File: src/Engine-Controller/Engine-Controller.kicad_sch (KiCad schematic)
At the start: 21 parts, among them J1 Jumper_NO, J2 Jumper_NO, P3 3220-20-0200-00, U1 STM32H750VBTx, Y1 ECS-240-18-33-JGN-TR

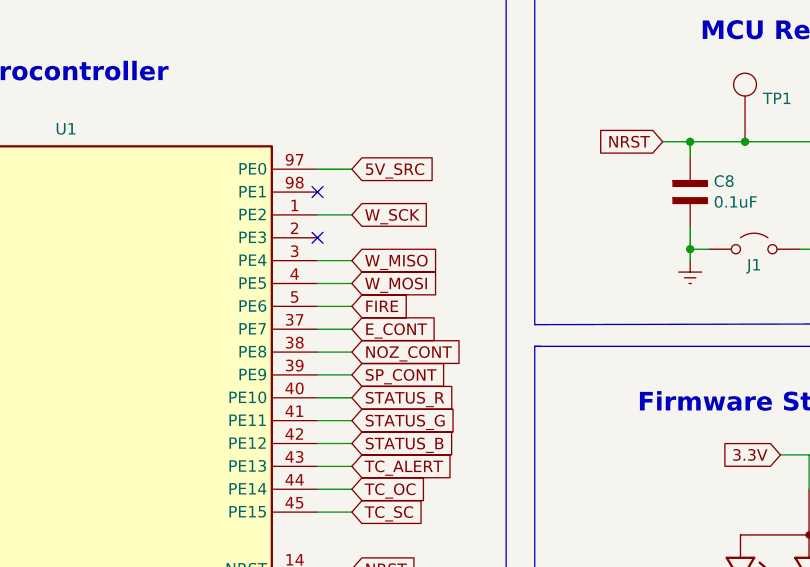
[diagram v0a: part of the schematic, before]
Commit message: completed rev 5.0 layout
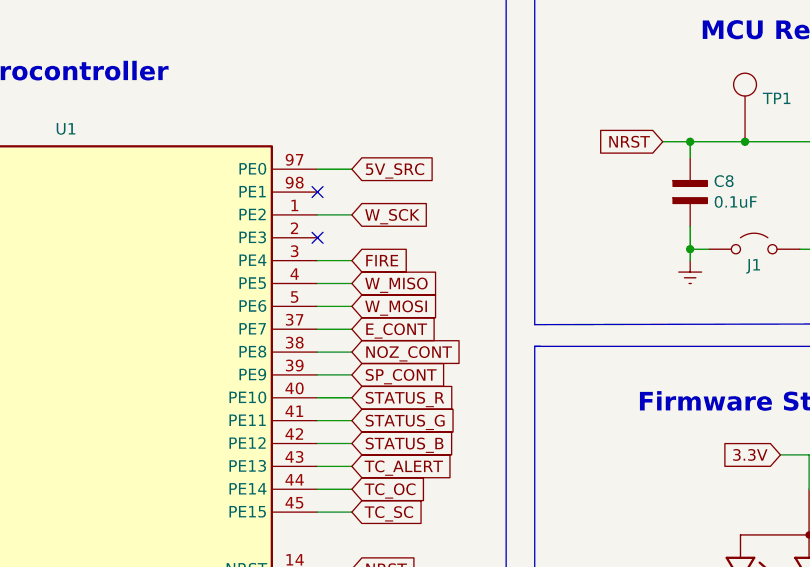
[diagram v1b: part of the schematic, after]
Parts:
- J1: footprint (none) -> Engine-Controller:Jumper-NO
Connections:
- net FIRE: now also U1.3 (PE4); no longer U1.5 (PE6)
- net W_MISO: now also U1.4 (PE5); no longer U1.3 (PE4)
- net W_MOSI: now also U1.5 (PE6); no longer U1.4 (PE5)
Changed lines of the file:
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@@
+    (stroke (width 0) (type default))
+  )
+  (polyline (pts (xy 172.085 59.055) (xy 172.085 116.205))
+    (stroke (width 0) (type default))
+  )
+  (wire (pts (xy 31.75 168.91) (xy 34.29 168.91))
+    (stroke (width 0) (type default))
+  )
+  (wire (pts (xy 91.44 44.45) (xy 95.25 44.45))
+    (stroke (width 0) (type default))
+  )
+  (wire (pts (xy 31.115 116.84) (xy 34.29 116.84))
+    (stroke (width 0) (type default))
+  )
+  (polyline (pts (xy 15.875 20.32) (xy 112.395 20.32))
+    (stroke (width 0) (type default))
+  )
+  (polyline (pts (xy 115.57 162.56) (xy 172.085 162.56))
+    (stroke (width 0) (type default))
+  )
+  (polyline (pts (xy 281.94 127) (xy 281.94 160.02))
+    (stroke (width 0) (type default))
+  )
+  (polyline (pts (xy 177.165 153.67) (xy 177.292 76.962))
+    (stroke (width 0) (type default))
+  )
+  (polyline (pts (xy 281.94 160.02) (xy 231.775 160.02))
+    (stroke (width 0) (type default))
+  )
+  (wire (pts (xy 31.75 158.75) (xy 34.29 158.75))
+    (stroke (width 0) (type default))
+  )
+  (wire (pts (xy 204.47 140.335) (xy 207.01 140.335))
+    (stroke (width 0) (type default))
+  )
+  (polyline (pts (xy 115.57 120.65) (xy 172.085 120.65))
+    (stroke (width 0) (type default))
+  )
+  (wire (pts (xy 204.47 147.955) (xy 204.47 145.415))
+    (stroke (width 0) (type default))
+  )
+  (wire (pts (xy 207.01 104.775) (xy 204.47 104.775))
+    (stroke (width 0) (type default))
+  )
+  (wire (pts (xy 91.44 62.23) (xy 95.25 62.23))
+    (stroke (width 0) (type default))
+  )
+  (wire (pts (xy 91.44 39.37) (xy 95.25 39.37))
+    (stroke (width 0) (type default))
+  )
+  (wire (pts (xy 264.16 150.495) (xy 264.16 152.4))
+    (stroke (width 0) (type default))
+  )
+  (wire (pts (xy 31.75 135.89) (xy 34.29 135.89))
+    (stroke (width 0) (type default))
+  )
+  (polyline (pts (xy 115.57 160.02) (xy 115.57 120.65))
+    (stroke (width 0) (type default))
+  )
+  (polyline (pts (xy 231.775 127) (xy 231.775 160.02))
+    (stroke (width 0) (type default))
+  )
+  (wire (pts (xy 204.47 120.015) (xy 207.01 120.015))
+    (stroke (width 0) (type default))
+  )
+  (wire (pts (xy 201.295 117.475) (xy 191.135 117.475))
+    (stroke (width 0) (type default))
+  )
+  (wire (pts (xy 31.115 127) (xy 34.29 127))
+    (stroke (width 0) (type default))
+  )
+  (polyline (pts (xy 172.085 116.205) (xy 115.57 116.205))
     (stroke (width 0) (type default))
   )
@@
     (stroke (width 0) (type default))
   )
-  (polyline (pts (xy 172.085 59.055) (xy 172.085 116.205))
-    (stroke (width 0) (type default))
-  )
-  (wire (pts (xy 31.75 168.91) (xy 34.29 168.91))
-    (stroke (width 0) (type default))
-  )
-  (wire (pts (xy 91.44 44.45) (xy 95.25 44.45))
-    (stroke (width 0) (type default))
-  )
-  (wire (pts (xy 31.115 116.84) (xy 34.29 116.84))
-    (stroke (width 0) (type default))
-  )
-  (polyline (pts (xy 15.875 20.32) (xy 112.395 20.32))
-    (stroke (width 0) (type default))
-  )
-  (polyline (pts (xy 115.57 162.56) (xy 172.085 162.56))
-    (stroke (width 0) (type default))
-  )
-  (polyline (pts (xy 281.94 127) (xy 281.94 160.02))
-    (stroke (width 0) (type default))
-  )
-  (polyline (pts (xy 177.165 153.67) (xy 177.292 76.962))
-    (stroke (width 0) (type default))
-  )
-  (polyline (pts (xy 281.94 160.02) (xy 231.775 160.02))
-    (stroke (width 0) (type default))
-  )
-  (wire (pts (xy 31.75 158.75) (xy 34.29 158.75))
-    (stroke (width 0) (type default))
-  )
-  (wire (pts (xy 204.47 140.335) (xy 207.01 140.335))
-    (stroke (width 0) (type default))
-  )
-  (polyline (pts (xy 115.57 120.65) (xy 172.085 120.65))
-    (stroke (width 0) (type default))
-  )
-  (wire (pts (xy 204.47 147.955) (xy 204.47 145.415))
-    (stroke (width 0) (type default))
-  )
-  (wire (pts (xy 207.01 104.775) (xy 204.47 104.775))
-    (stroke (width 0) (type default))
-  )
-  (wire (pts (xy 91.44 62.23) (xy 95.25 62.23))
-    (stroke (width 0) (type default))
-  )
-  (wire (pts (xy 91.44 39.37) (xy 95.25 39.37))
-    (stroke (width 0) (type default))
-  )
-  (wire (pts (xy 264.16 150.495) (xy 264.16 152.4))
-    (stroke (width 0) (type default))
-  )
-  (wire (pts (xy 31.75 135.89) (xy 34.29 135.89))
-    (stroke (width 0) (type default))
-  )
-  (polyline (pts (xy 115.57 160.02) (xy 115.57 120.65))
-    (stroke (width 0) (type default))
-  )
-  (polyline (pts (xy 231.775 127) (xy 231.775 160.02))
-    (stroke (width 0) (type default))
-  )
-  (wire (pts (xy 204.47 120.015) (xy 207.01 120.015))
-    (stroke (width 0) (type default))
-  )
-  (wire (pts (xy 201.295 117.475) (xy 191.135 117.475))
-    (stroke (width 0) (type default))
-  )
-  (wire (pts (xy 31.115 127) (xy 34.29 127))
-    (stroke (width 0) (type default))
-  )
-  (polyline (pts (xy 172.085 116.205) (xy 115.57 116.205))
-    (stroke (width 0) (type default))
-  )
   (wire (pts (xy 31.75 163.83) (xy 34.29 163.83))
     (stroke (width 0) (type default))
@@
     (stroke (width 0) (type default))
   )
+  (wire (pts (xy 91.44 49.53) (xy 95.25 49.53))
+    (stroke (width 0) (type default))
+  )
   (wire (pts (xy 31.115 77.47) (xy 34.29 77.47))
     (stroke (width 0) (type default))
@@
     (stroke (width 0) (type default))
   )
-  (wire (pts (xy 91.44 49.53) (xy 95.25 49.53))
-    (stroke (width 0) (type default))
-  )
   (wire (pts (xy 91.44 110.49) (xy 95.25 110.49))
     (stroke (width 0) (type default))
@@
     (stroke (width 0) (type default))
   )
+  (wire (pts (xy 91.44 54.61) (xy 95.25 54.61))
+    (stroke (width 0) (type default))
+  )
   (wire (pts (xy 148.59 177.8) (xy 151.13 177.8))
     (stroke (width 0) (type default))
@@
   )
   (polyline (pts (xy 115.57 116.205) (xy 115.57 59.055))
-    (stroke (width 0) (type default))
-  )
-  (wire (pts (xy 91.44 54.61) (xy 95.25 54.61))
     (stroke (width 0) (type default))
   )
@@
     )
   )
-  (global_label "W_MISO" (shape input) (at 95.25 49.53 0) (fields_autoplaced)
-    (effects (font (size 1.27 1.27)) (justify left))
-    (property "Intersheetrefs" "${INTERSHEET_REFS}" (at 104.5894 49.6094 0)
-      (effects (font (size 1.27 1.27)) (justify left) hide)
-    )
-  )
-  (global_label "W_MOSI" (shape input) (at 95.25 52.07 0) (fields_autoplaced)
+  (global_label "W_MISO" (shape input) (at 95.25 52.07 0) (fields_autoplaced)
     (effects (font (size 1.27 1.27)) (justify left))
     (property "Intersheetrefs" "${INTERSHEET_REFS}" (at 104.5894 52.1494 0)
@@
     )
   )
+  (global_label "W_MOSI" (shape input) (at 95.25 54.61 0) (fields_autoplaced)
+    (effects (font (size 1.27 1.27)) (justify left))
+    (property "Intersheetrefs" "${INTERSHEET_REFS}" (at 104.5894 54.6894 0)
+      (effects (font (size 1.27 1.27)) (justify left) hide)
+    )
+  )
   (global_label "SWDIO" (shape input) (at 31.115 124.46 180) (fields_autoplaced)
     (effects (font (size 1.27 1.27)) (justify right))
@@
     )
   )
-  (global_label "FIRE" (shape input) (at 95.25 54.61 0) (fields_autoplaced)
-    (effects (font (size 1.27 1.27)) (justify left))
-    (property "Intersheetrefs" "${INTERSHEET_REFS}" (at -43.18 5.08 0)
+  (global_label "FIRE" (shape input) (at 95.25 49.53 0) (fields_autoplaced)
+    (effects (font (size 1.27 1.27)) (justify left))
+    (property "Intersheetrefs" "${INTERSHEET_REFS}" (at -43.18 0 0)
       (effects (font (size 1.27 1.27)) hide)
     )
@@
       (effects (font (size 1.27 1.27)) hide)
     )
-    (property "Footprint" "" (at 139.954 48.26 0)
-      (effects (font (size 1.27 1.27)) hide)
-    )
+    (property "Footprint" "Engine-Controller:Jumper-NO" (at 139.954 48.26 0)
+      (effects (font (size 1.27 1.27)) hide)
+    )
